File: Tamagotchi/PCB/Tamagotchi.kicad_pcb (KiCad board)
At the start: 2 copper layers, 70.1 x 85.3 mm, 21 parts, among them SW1 SW_Push, SW2 SW_Push, SW3 SW_Push, SW4 SW_Push, SW5 SW_SPDT, U1 ESP32-C3-SuperMini, U2 SSD1306

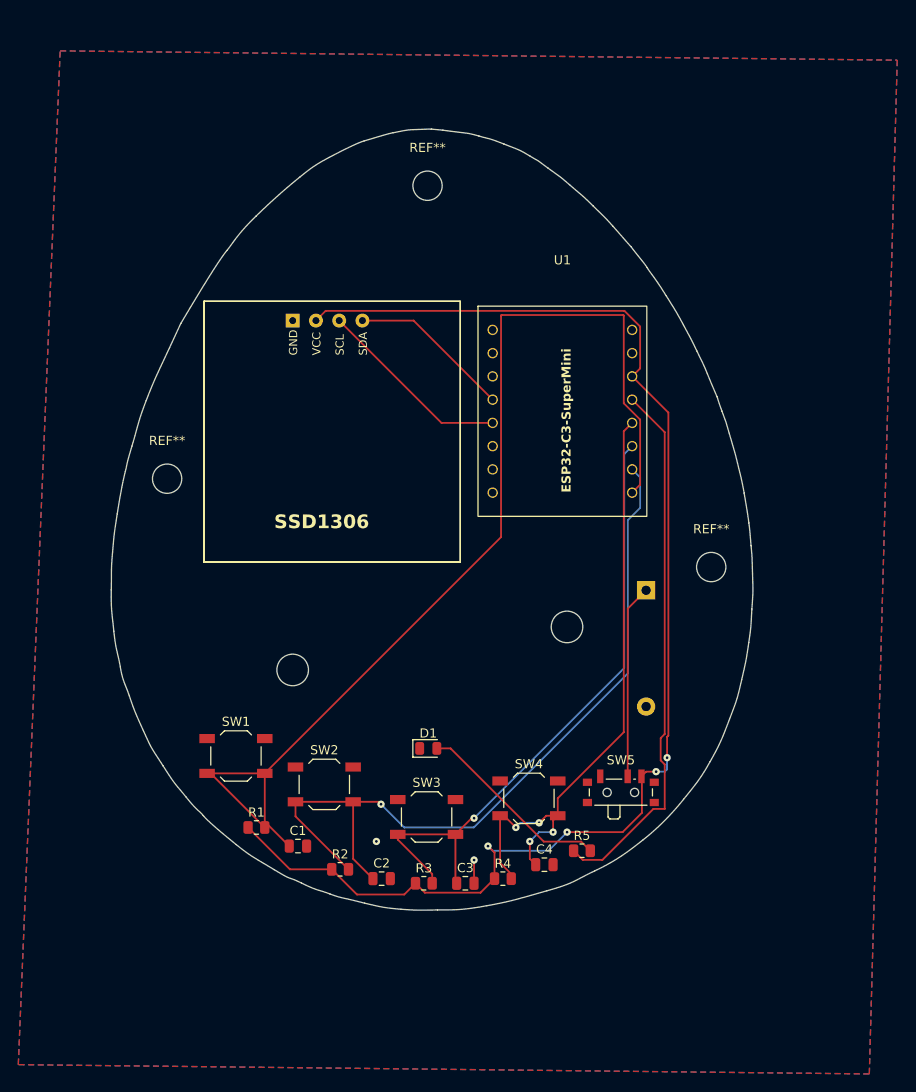
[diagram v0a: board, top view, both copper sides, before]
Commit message: updated Tamagotchi
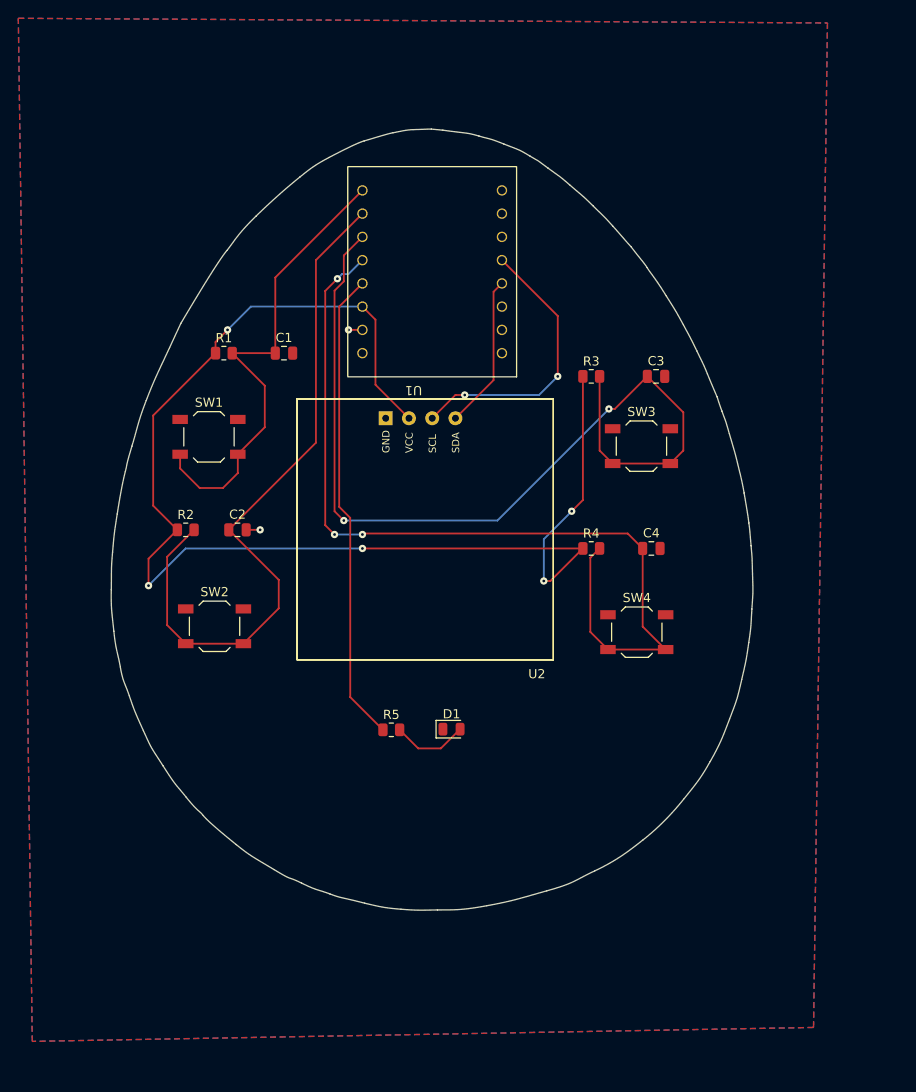
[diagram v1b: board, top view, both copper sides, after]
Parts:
- removed BT1: Battery_Cell, Battery:BatteryHolder_Keystone_2468_2xAAA
- removed REF** (x3): MountingHole_3.2mm_M3, MountingHole:MountingHole_3.2mm_M3
- removed SW5: SW_SPDT, Button_Switch_SMD:SW_SPDT_PCM12
- moved C3 59.2 mm to (170.2, 87.9)
- moved R3 58.3 mm to (163.2, 87.9)
- moved C1 53.9 mm to (129.6, 85.3)
- moved R1 51.9 mm to (123.0, 85.3)
- moved SW3 46.8 mm to (168.7, 95.5)
- moved C2 41.2 mm to (124.5, 104.6)
- moved R2 40.7 mm to (118.9, 104.6)
- moved R4 37.3 mm to (163.2, 106.7)
- moved C4 36.5 mm to (169.7, 106.7)
- moved SW1 35.0 mm to (121.4, 94.5)
- moved R5 24.7 mm to (141.3, 126.5)
- moved SW4 21.6 mm to (168.1, 115.8)
- moved SW2 21.0 mm to (122.0, 115.2)
- moved U1 20.8 mm to (145.8, 76.5), turned to 180 degrees
- moved U2 14.7 mm to (144.5, 101.3)
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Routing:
- net Net-(U1-GPIO0): track 118.7 -> 51.6 mm
- net Net-(U1-GPIO2): track 69.2 -> 100.5 mm, vias 1 -> 2
- net Net-(U1-GPIO3): track 68.8 -> 97.5 mm, vias 4 -> 3
- net Net-(BT1-+): track 21.2 -> 0.00 mm
- net Net-(D1-A): track 21.4 -> 8.32 mm
- net Net-(U1-GPIO9): track 21.4 -> 30.8 mm, vias 0 -> 2
- net Net-(U1-GPIO1): track 86.7 -> 77.7 mm, vias 1 -> 0
- net Net-(U1-GPIO4): track 59.2 -> 51.8 mm
- net Net-(U2-VCC): track 148.2 -> 142.8 mm, vias 4 -> 5
- net Net-(U1-GPIO8): track 17.8 -> 16.8 mm
- net GND: track 2.54 -> 3.05 mm
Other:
- board text removed: "ESP32-C3-SuperMini"
- board text removed: "SSD1306"
